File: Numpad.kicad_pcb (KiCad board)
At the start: 2 copper layers, 82.6 x 127 mm, 70 parts, among them J2 USB_C_Receptacle_USB2.0, U1 SRV05-4, U2 STM32F103C8Tx, U3 XC6206PxxxMR, Y1 8MHz

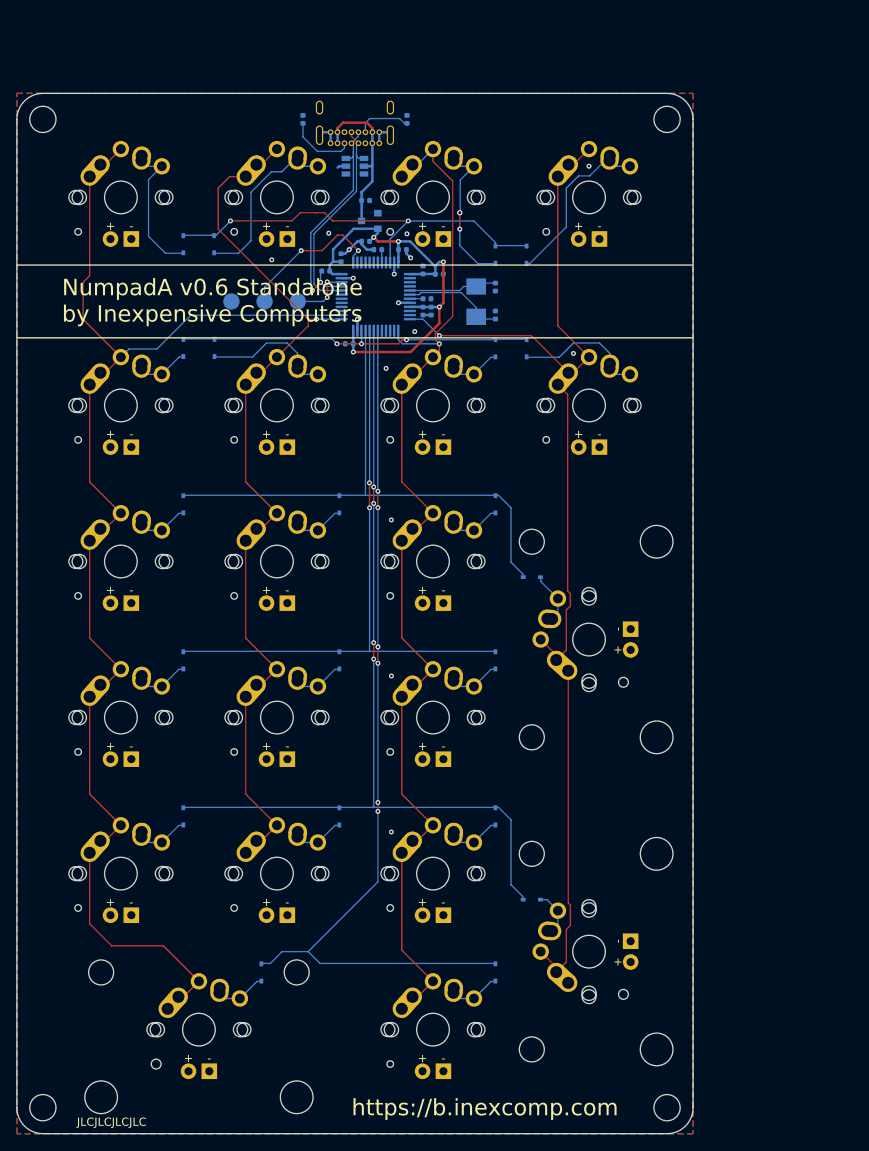
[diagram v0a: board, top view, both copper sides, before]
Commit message: v0.9pre
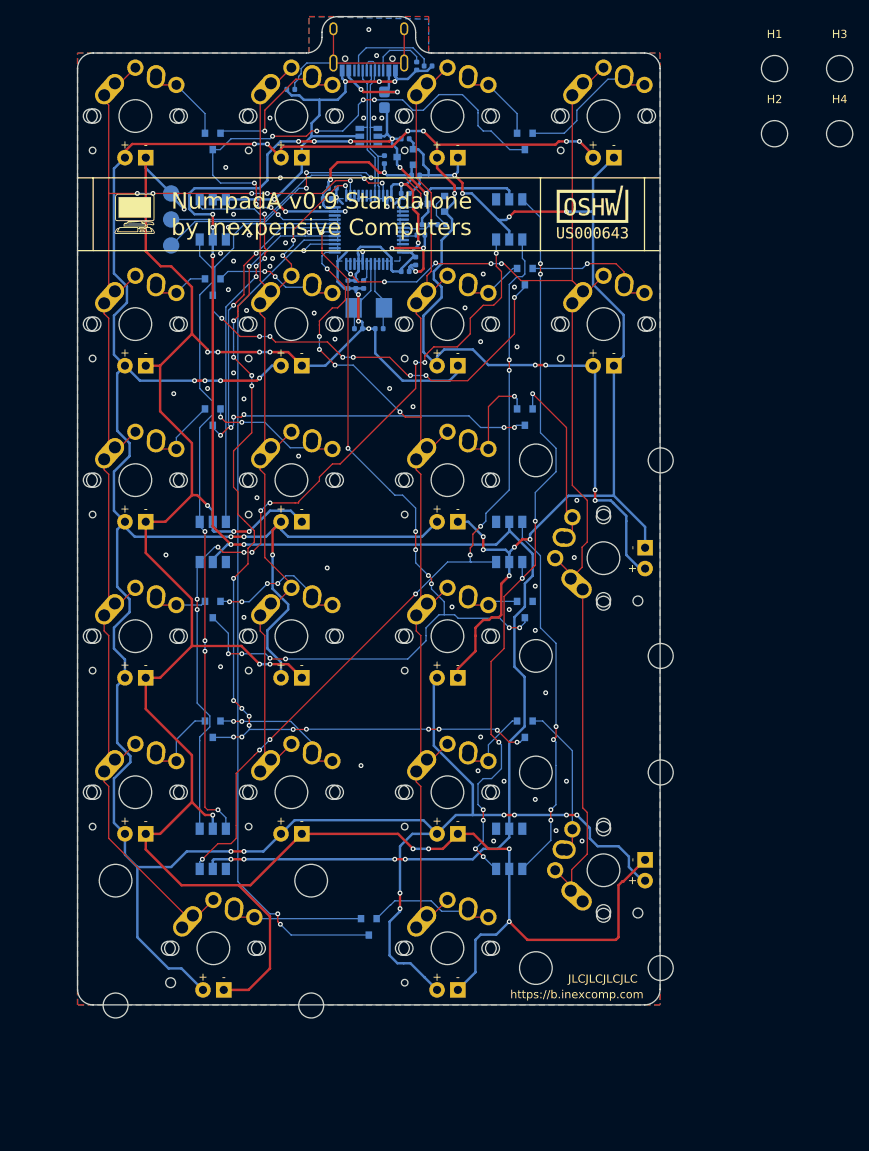
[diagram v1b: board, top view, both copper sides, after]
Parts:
- removed C1, C2, C3, C4, C6: 100nf, Capacitor_SMD:C_0402_1005Metric
- removed C5: 1uf, Capacitor_SMD:C_0402_1005Metric
- removed D_0, D_1, D_2, D_3, D_4, D_5, D_6, D_7, D_8, D_9, D_BKSP1, D_DOT1, D_ENTER1, D_ESC1, D_FN1, D_MINUS1, D_NUMLK1, D_PLUS1, D_SLASH1, D_STAR1, D_TAB1: 1N4148WS, Diode_SMD:D_SOD-323
- removed J2: USB_C_Receptacle_USB2.0, Connector_USB:USB_C_Receptacle_GCT_USB4085
- removed R4: 1.5K, Resistor_SMD:R_0402_1005Metric
- added C13: 20pf, Capacitor_SMD:C_0402_1005Metric, B.Cu at (80.6, 66.7)
- added C14: 100nf, Capacitor_SMD:C_0402_1005Metric, B.Cu at (81.3, 61.3)
- added C15: 100nf, Capacitor_SMD:C_0402_1005Metric, B.Cu at (87.6, 58.4)
- added C16: 1uf, Capacitor_SMD:C_0402_1005Metric, B.Cu at (79.4, 61.3)
- added C17: 100nf, Capacitor_SMD:C_0402_1005Metric, B.Cu at (80.3, 61.3)
- added C18: 100nf, Capacitor_SMD:C_0402_1005Metric, B.Cu at (77.5, 49.5)
- added D1: WS2813, LED_SMD:LED_WS2812_PLCC6_5.0x5.0mm_P1.6mm, B.Cu at (62.9, 53.3)
- added D10: BAT54C, Package_TO_SOT_SMD:SOT-23, B.Cu at (62.9, 101.0)
- added D11: BAT54C, Package_TO_SOT_SMD:SOT-23, B.Cu at (62.9, 115.6)
- added D12: BAT54C, Package_TO_SOT_SMD:SOT-23, B.Cu at (81.9, 139.7)
- added D13: BAT54C, Package_TO_SOT_SMD:SOT-23, B.Cu at (101.0, 43.8)
- added D14: BAT54C, Package_TO_SOT_SMD:SOT-23, B.Cu at (101.0, 60.3)
- added D15: BAT54C, Package_TO_SOT_SMD:SOT-23, B.Cu at (101.0, 77.5)
- added D16: BAT54C, Package_TO_SOT_SMD:SOT-23, B.Cu at (101.0, 101.0)
- added D17: BAT54C, Package_TO_SOT_SMD:SOT-23, B.Cu at (101.0, 115.6)
- added D2: WS2813, LED_SMD:LED_WS2812_PLCC6_5.0x5.0mm_P1.6mm, B.Cu at (99.1, 53.3)
- added D3: WS2813, LED_SMD:LED_WS2812_PLCC6_5.0x5.0mm_P1.6mm, B.Cu at (62.9, 92.7)
- added D4: WS2813, LED_SMD:LED_WS2812_PLCC6_5.0x5.0mm_P1.6mm, B.Cu at (99.1, 92.7)
- added D5: WS2813, LED_SMD:LED_WS2812_PLCC6_5.0x5.0mm_P1.6mm, B.Cu at (62.9, 130.2)
- added D6: WS2813, LED_SMD:LED_WS2812_PLCC6_5.0x5.0mm_P1.6mm, B.Cu at (99.1, 130.2)
- added D7: BAT54C, Package_TO_SOT_SMD:SOT-23, B.Cu at (62.9, 43.8)
- added D8: BAT54C, Package_TO_SOT_SMD:SOT-23, B.Cu at (62.9, 61.6)
- added D9: BAT54C, Package_TO_SOT_SMD:SOT-23, B.Cu at (62.9, 77.5)
- added F1: SMD0805P050TF, Fuse:Fuse_0805_2012Metric_Castellated, B.Cu at (83.8, 38.7)
- added G***: LOGO, Logo:inexcomplogo1, F.Cu at (53.3, 52.7)
- added G***: LOGO, Logo:OSHWMark, F.Cu at (109.2, 52.7)
- added J1: USB_C_Receptacle_USB2.0, Connector_USB:USB_C_Receptacle_HRO_TYPE-C-31-M-12, B.Cu at (81.9, 31.1)
- added Q1: AO3401A, Package_TO_SOT_SMD:SOT-23, B.Cu at (90.2, 51.4)
- added R11: 10k, Resistor_SMD:R_0402_1005Metric, B.Cu at (88.3, 55.2)
- added R12: 1.5K, Resistor_SMD:R_0402_1005Metric, B.Cu at (83.8, 46.0)
- added R13: 5.1K, Resistor_SMD:R_0402_1005Metric, B.Cu at (89.2, 34.6)
- added R14: 5.1K, Resistor_SMD:R_0402_1005Metric, B.Cu at (87.8, 34.6)
- C10, C7: value 100nf -> 1uf
- C11: value 1uf -> 100nf
- C12: value 1uf -> 20pf
- C8, C9: value 20pf -> 100nf
- R1: value 10k -> 10K
- R2: value 5.1K -> 150R
- R3: value 5.1K -> 1M
- SW_0, SW_ENTER1, SW_PLUS1: footprint Keebio-Parts:MX-Alps-Choc-2U -> Keebio-Parts:MX-Alps-Choc-2U-StabFlip
- U1: value SRV05-4 -> STM32F103C8Tx; footprint Package_TO_SOT_SMD:SOT-23-6 -> Package_QFP:LQFP-48_7x7mm_P0.5mm
- U2: value STM32F103C8Tx -> XC6206PxxxMR; footprint Package_QFP:LQFP-48_7x7mm_P0.5mm -> Package_TO_SOT_SMD:SOT-23
- U3: value XC6206PxxxMR -> SRV05-4; footprint Package_TO_SOT_SMD:SOT-23 -> Package_TO_SOT_SMD:SOT-23-6
- moved H3 159.9 mm to (139.4, 34.9)
- moved H4 120.8 mm to (139.4, 42.9)
- moved H1 89.5 mm to (131.4, 34.9)
- moved C9 25.0 mm to (76.8, 50.8), turned to 180 degrees
- moved R2 21.3 mm to (90.8, 54.0), turned to 180 degrees
- moved SIO1 18.4 mm to (57.8, 53.3), turned to 270 degrees
- moved U2 17.4 mm to (86.4, 45.7)
- moved C7 17.0 mm to (86.4, 43.5)
- moved C10 15.1 mm to (87.6, 47.9)
- moved GND1 15.1 mm to (57.8, 50.2), turned to 270 degrees
- moved R3 14.6 mm to (72.4, 37.5), turned to 180 degrees
- moved SCK1 13.3 mm to (57.8, 56.5), turned to 270 degrees
- moved H2 13.2 mm to (131.4, 42.9)
- moved Y1 13.1 mm to (81.9, 64.1), turned to 0 degrees
- moved C8 11.2 mm to (86.4, 59.7), turned to 180 degrees
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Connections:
- net LED_PWR renamed LED_MATRIX
- C10 pad 1: NRST -> VBAT
- C11 pad 2: +5V -> VBAT
- C12 pad 1: VBAT -> PD0
- C7 pad 2: VBAT -> +5V
- C8 pad 1: PD0 -> GND
- C8 pad 2: GND -> VBAT
- C9 pad 1: PD1 -> GND
- C9 pad 2: GND -> VBAT
- R1 pad 1: BOOT0 -> +5V
- R1 pad 2: GND -> LED_CONTROL
- R2 pad 1: /CC1 -> Net-(Q1-Pad1)
- R2 pad 2: GND -> LED_CONTROL
- R3 pad 1: GND -> Net-(J1-PadS1)
- R3 pad 2: /CC2 -> GND
- U1 pad 1: (no net) -> VBAT
- U1 pad 2: GND -> (no net)
- U1 pad 3: DA+ -> (no net)
- U1 pad 4: DA- -> (no net)
- U1 pad 5: +5V -> PD0
- U1 pad 6: (no net) -> PD1
- U2 pad 1: VBAT -> GND
- U2 pad 2: (no net) -> VBAT
- U2 pad 3: (no net) -> +5V
- U3 pad 1: GND -> (no net)
- U3 pad 2: VBAT -> GND
- U3 pad 3: +5V -> DA-
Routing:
- net GND: track 19.9 -> 541.1 mm, vias 16 -> 92
- net LED_MATRIX: track 0.00 -> 461.7 mm, vias 0 -> 26
- net +5V: track 19.6 -> 224.8 mm, vias 0 -> 15
- net Net-(D2-Pad4): track 0.00 -> 99.5 mm, vias 0 -> 8
- net Net-(D2-Pad6): track 0.00 -> 98.1 mm, vias 0 -> 10
- net Net-(D2-Pad3): track 0.00 -> 92.8 mm, vias 0 -> 9
- net Net-(D1-Pad3): track 0.00 -> 76.6 mm, vias 0 -> 4
- net BL_CONTROL: track 0.00 -> 57.9 mm, vias 0 -> 5
- net Net-(D4-Pad3): track 0.00 -> 46.0 mm, vias 0 -> 4
- net row2: track 44.0 -> 72.4 mm, vias 3 -> 8
- net col3: track 122.9 -> 149.0 mm, vias 1 -> 5
- net Net-(J1-PadS1): track 0.00 -> 24.1 mm
- net row4: track 77.3 -> 101.3 mm, vias 2 -> 12
- net SWDIO: track 7.49 -> 30.0 mm
- net SWDCLK: track 18.3 -> 40.0 mm, vias 2 -> 4
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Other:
- board size 82.6 x 127 mm -> 71.1 x 120.6 mm
- board text added: "NumpadA v0.9 Standalone by Inexpensive Computers"
- board text removed: "NumpadA v0.6 Standalone by Inexpensive Computers"
